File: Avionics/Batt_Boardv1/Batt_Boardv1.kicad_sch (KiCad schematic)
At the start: 13 parts

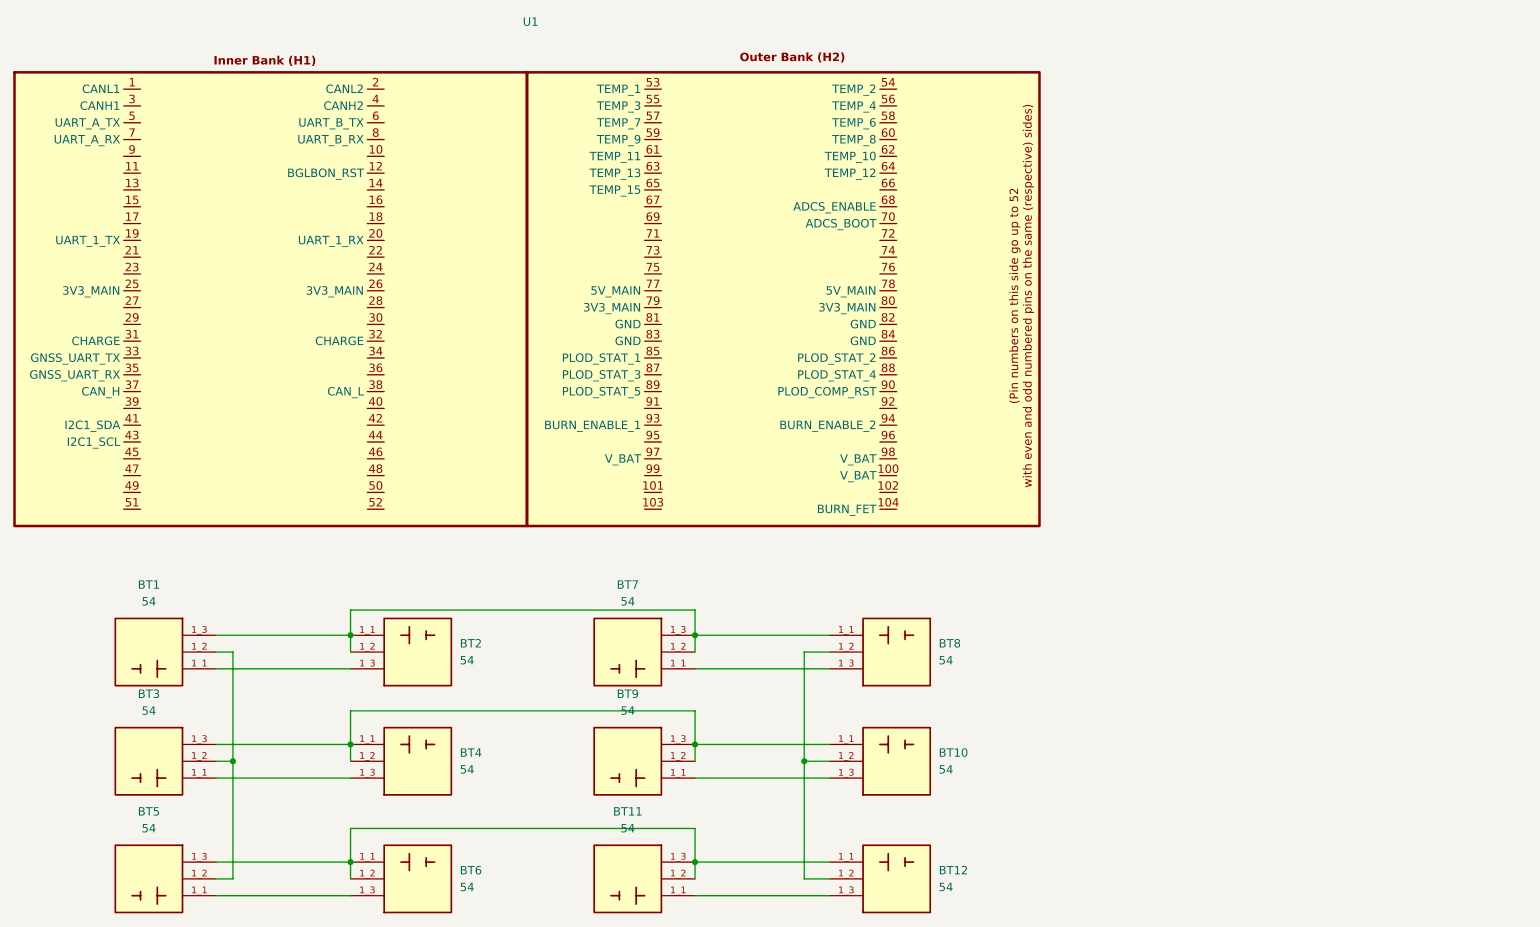
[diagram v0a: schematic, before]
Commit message: yippie
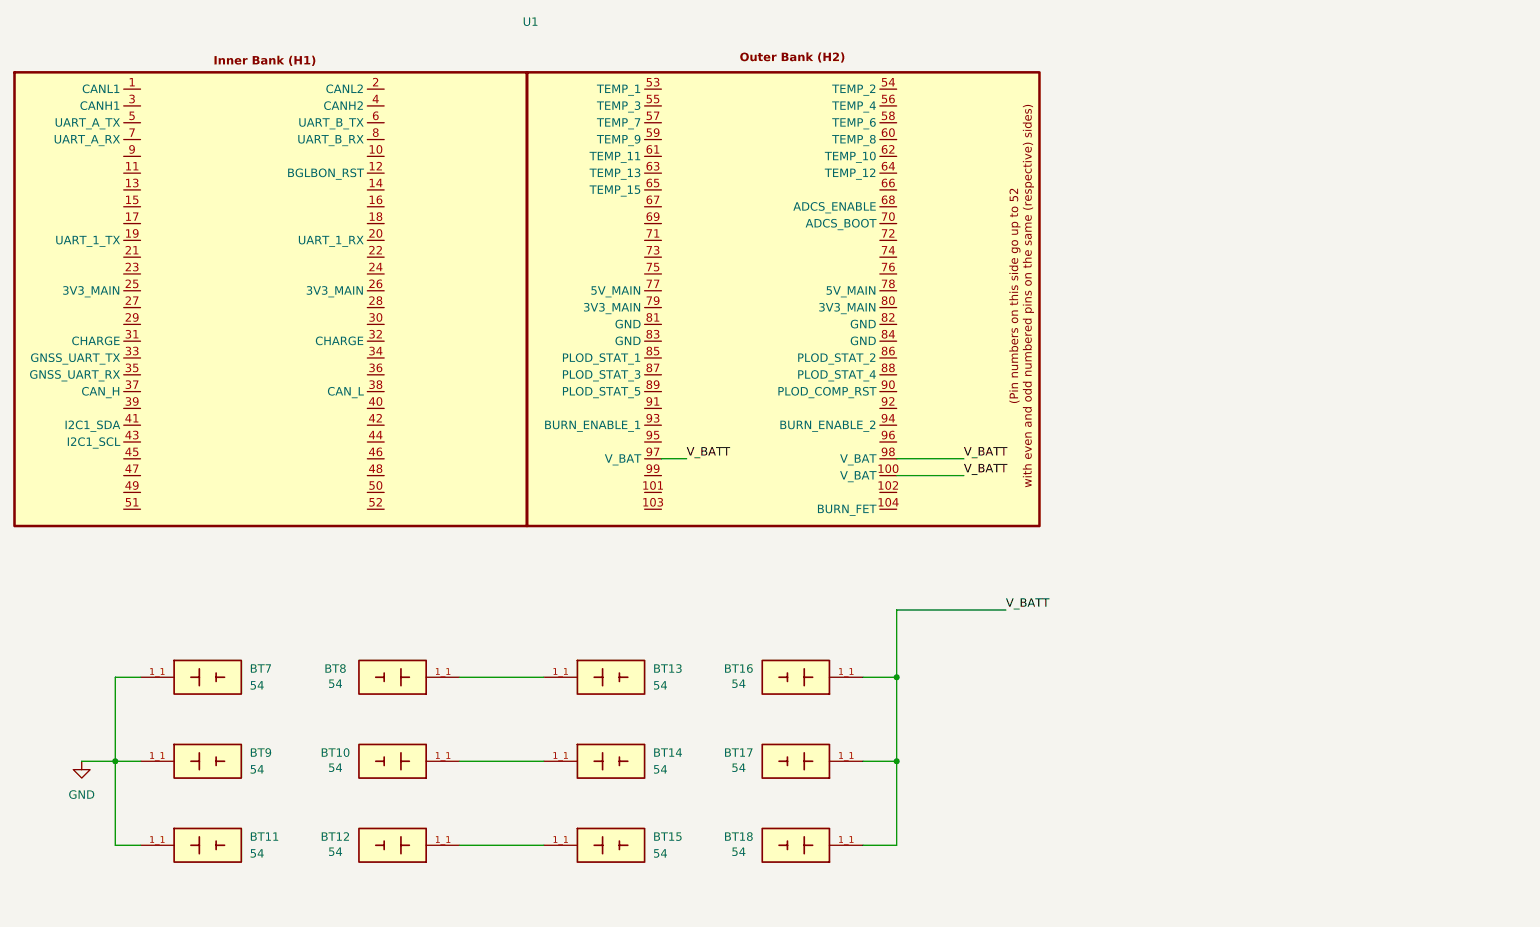
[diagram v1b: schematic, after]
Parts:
- removed BT1, BT10, BT11, BT12, BT2, BT3, BT4, BT5, BT6, BT7, BT8, BT9: 54, 54:BAT_54, symbol Battery Holder:54
- added BT10, BT11, BT12, BT13, BT14, BT15, BT16, BT17, BT18, BT7, BT8, BT9: 54, Battery 54:BAT_254TR, symbol 54 -- Battery clips:54
- U1: footprint GPIO2_7 -> PC104:PC104ConnectorFootprint (1)
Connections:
- net V_BATT: now reaches U1.100 (V_BAT)
- net V_BATT: now also U1.97 (V_BAT), U1.98 (V_BAT), BT16.1_1, BT17.1_1, BT18.1_1
- new net: BT13.1_1, BT8.1_1
- new net: BT10.1_1, BT14.1_1
- new net: BT12.1_1, BT15.1_1
- new net GND: BT11.1_1, BT7.1_1, BT9.1_1

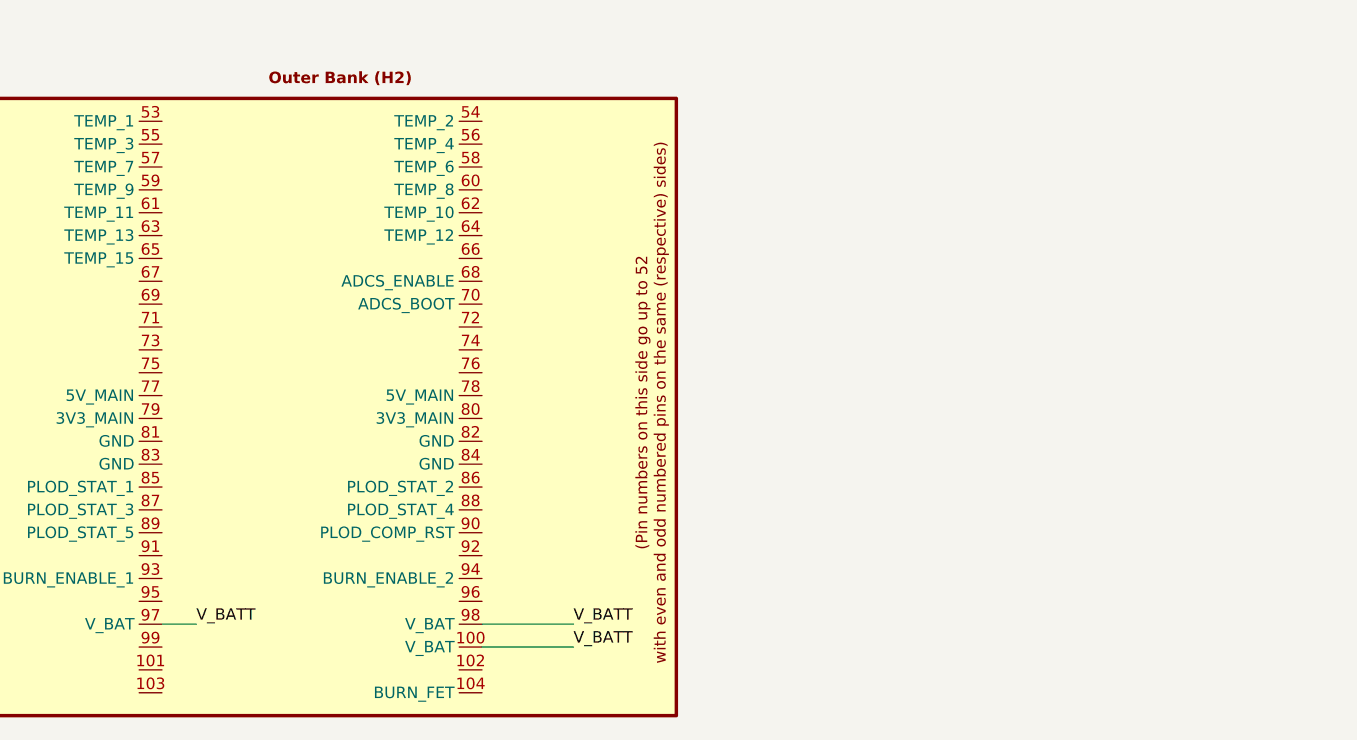
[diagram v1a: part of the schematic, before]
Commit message: need to fic tracks
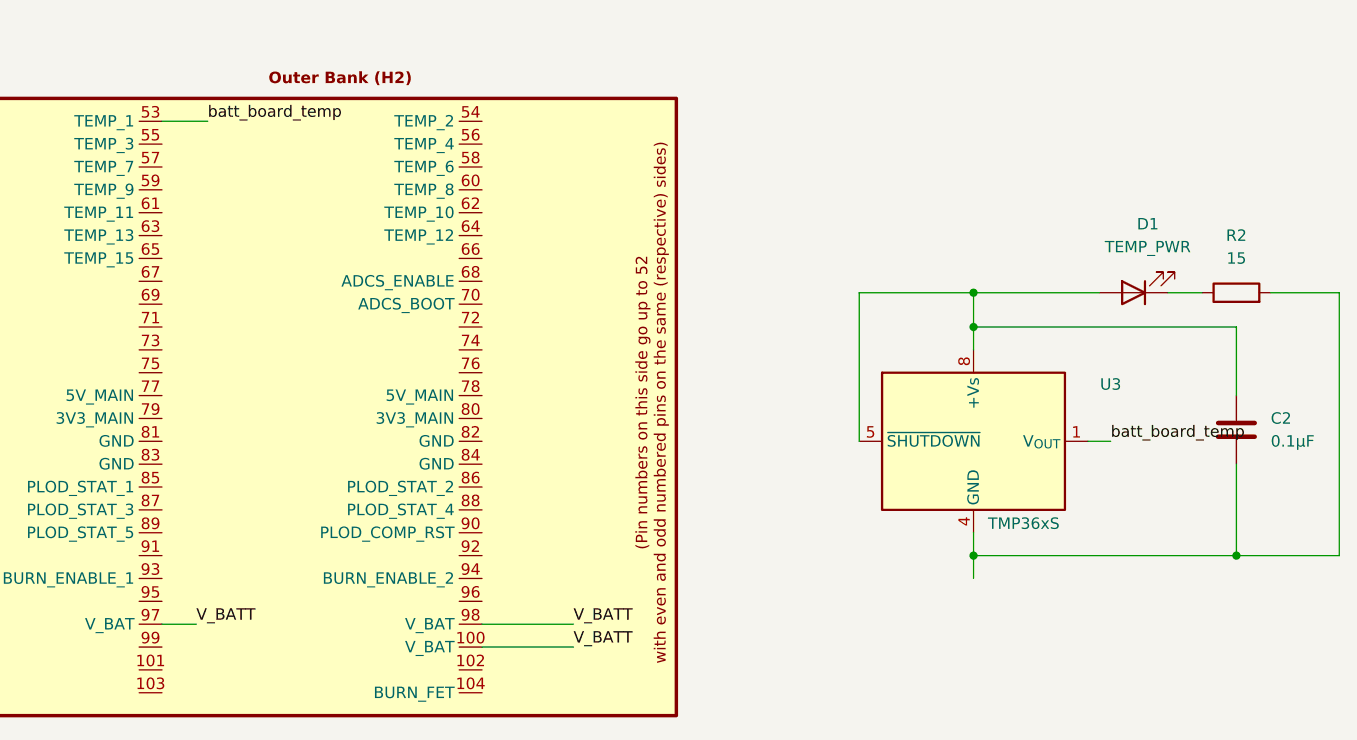
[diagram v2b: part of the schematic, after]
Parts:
- added C2: 0.1µF, Capacitor_SMD:C_0805_2012Metric, symbol Device:C
- added D1: TEMP_PWR, LED_SMD:LED_0805_2012Metric, symbol Device:LED
- added R2: 15, Resistor_SMD:R_0805_2012Metric, symbol Device:R
- added U3: TMP36xS, Package_SO:SOIC-8_3.9x4.9mm_P1.27mm, symbol Sensor_Temperature:TMP36xS
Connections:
- net batt_board_temp: now reaches U1.53 (TEMP_1)
- net batt_board_temp: now also U3.1 (V_{OUT})
- new net: D1.1 (K), R2.1
- new net: C2.2, R2.2, U3.4 (GND)
- new net: C2.1, D1.2 (A), U3.5 (~{SHUTDOWN}), U3.8 (+Vs)
